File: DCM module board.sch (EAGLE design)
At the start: 2 parts

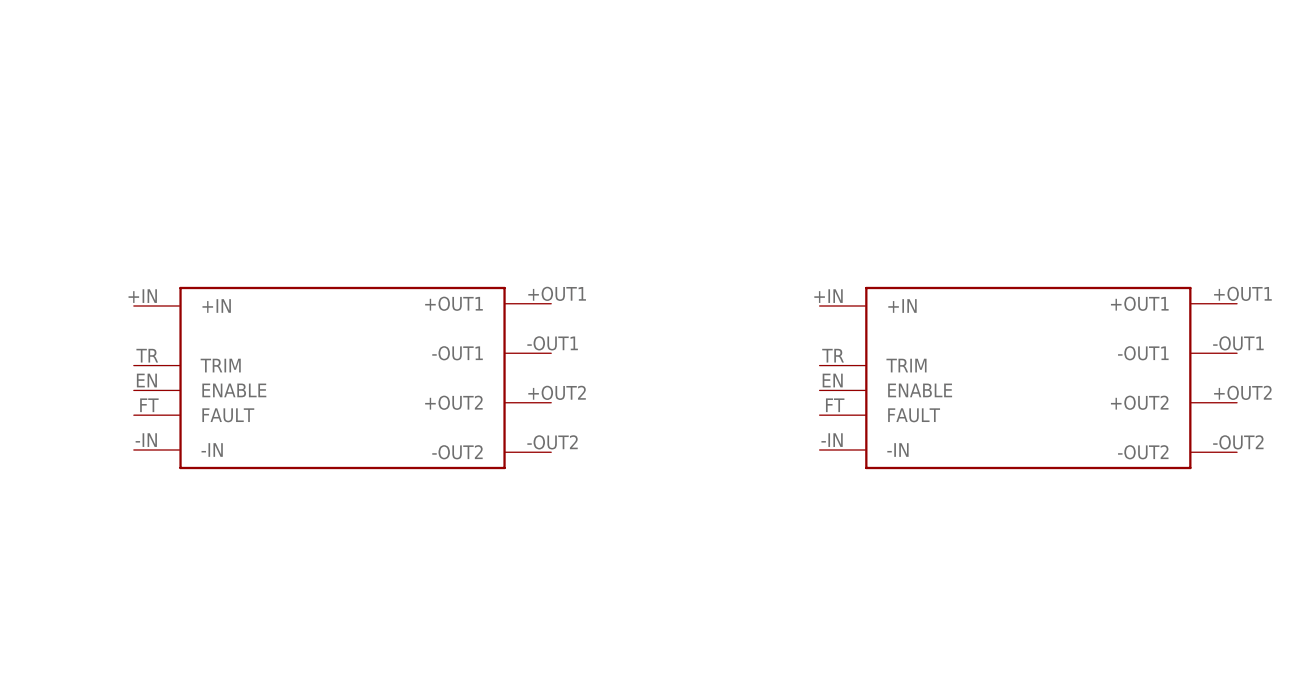
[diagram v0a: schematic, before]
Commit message: Add files via upload
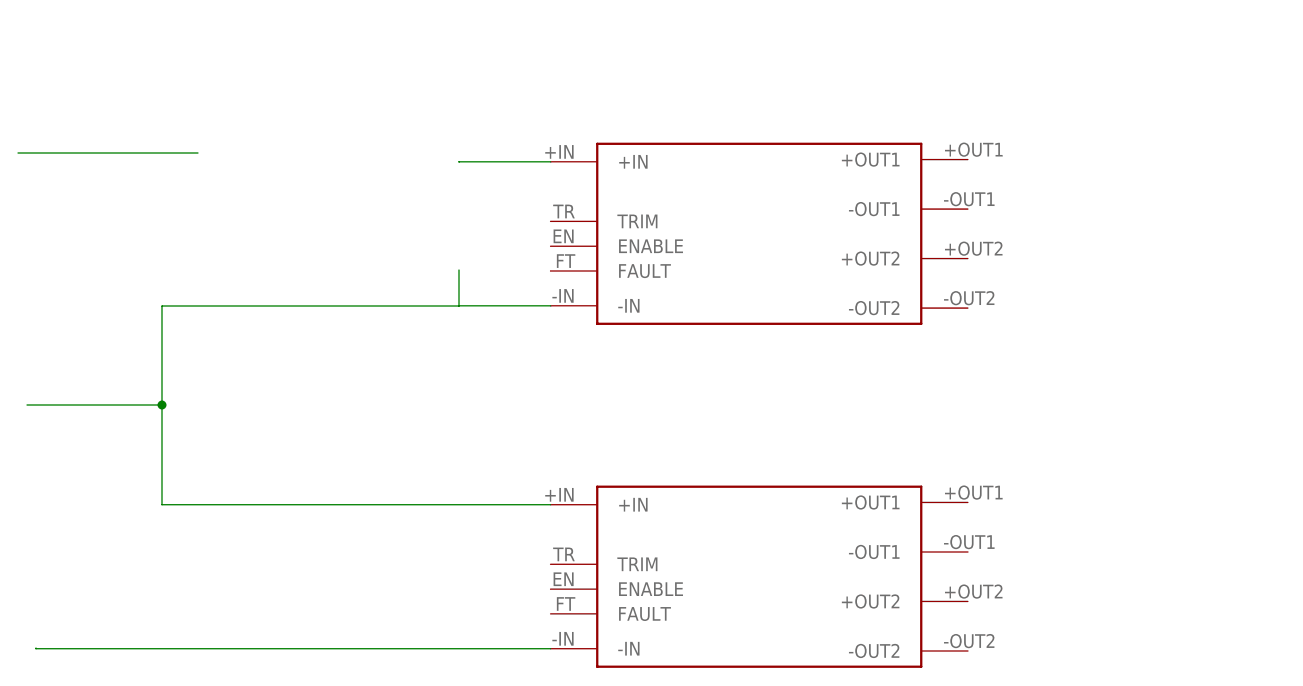
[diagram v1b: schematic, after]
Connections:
- new net N$1: U$1.+IN
- new net N$3: U$1.-IN
- new net N$4: U$2.+IN
- new net N$5: U$2.-IN
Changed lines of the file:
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@@
 <setting verticaltext="up"/>
 </settings>
-<grid distance="0.1" unitdist="inch" unit="inch" style="lines" multiple="1" display="no" altdistance="0.01" altunitdist="inch" altunit="inch"/>
+<grid distance="1" unitdist="mm" unit="mm" style="lines" multiple="1" display="yes" altdistance="0.01" altunitdist="inch" altunit="mm"/>
 <layers>
 <layer number="1" name="Top" color="4" fill="1" visible="no" active="no"/>
@@
 </plain>
 <instances>
-<instance part="U$1" gate="G$1" x="-27.94" y="0" smashed="yes"/>
-<instance part="U$2" gate="G$1" x="48.26" y="0" smashed="yes"/>
+<instance part="U$1" gate="G$1" x="18.36" y="16.02" smashed="yes"/>
+<instance part="U$2" gate="G$1" x="18.36" y="-22.08" smashed="yes"/>
 </instances>
 <busses>
 </busses>
 <nets>
+<net name="N$1" class="0">
+<segment>
+<pinref part="U$1" gate="G$1" pin="+IN"/>
+<wire x1="-4.83" y1="24.02" x2="-15" y2="24.02" width="0.1524" layer="91"/>
+<wire x1="-15" y1="24.02" x2="-15" y2="24" width="0.1524" layer="91"/>
+</segment>
+</net>
+<net name="N$2" class="0">
+<segment>
+<wire x1="-44" y1="25" x2="-64" y2="25" width="0.1524" layer="91"/>
+</segment>
+</net>
+<net name="N$3" class="0">
+<segment>
+<pinref part="U$1" gate="G$1" pin="-IN"/>
+<wire x1="-4.83" y1="8.02" x2="-15" y2="8.02" width="0.1524" layer="91"/>
+<wire x1="-15" y1="8.02" x2="-15" y2="12" width="0.1524" layer="91"/>
+</segment>
+</net>
+<net name="N$4" class="0">
+<segment>
+<wire x1="-15" y1="8" x2="-48" y2="8" width="0.1524" layer="91"/>
+<wire x1="-48" y1="8" x2="-48" y2="-3" width="0.1524" layer="91"/>
+<pinref part="U$2" gate="G$1" pin="+IN"/>
+<wire x1="-48" y1="-3" x2="-48" y2="-14.08" width="0.1524" layer="91"/>
+<wire x1="-48" y1="-14.08" x2="-4.83" y2="-14.08" width="0.1524" layer="91"/>
+<wire x1="-48" y1="-3" x2="-63" y2="-3" width="0.1524" layer="91"/>
+<junction x="-48" y="-3"/>
+</segment>
+</net>
+<net name="N$5" class="0">
+<segment>
+<pinref part="U$2" gate="G$1" pin="-IN"/>
+<wire x1="-4.83" y1="-30.08" x2="-62" y2="-30.08" width="0.1524" layer="91"/>
+<wire x1="-62" y1="-30.08" x2="-62" y2="-30" width="0.1524" layer="91"/>
+</segment>
+</net>
 </nets>
 </sheet>

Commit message: Add files via upload
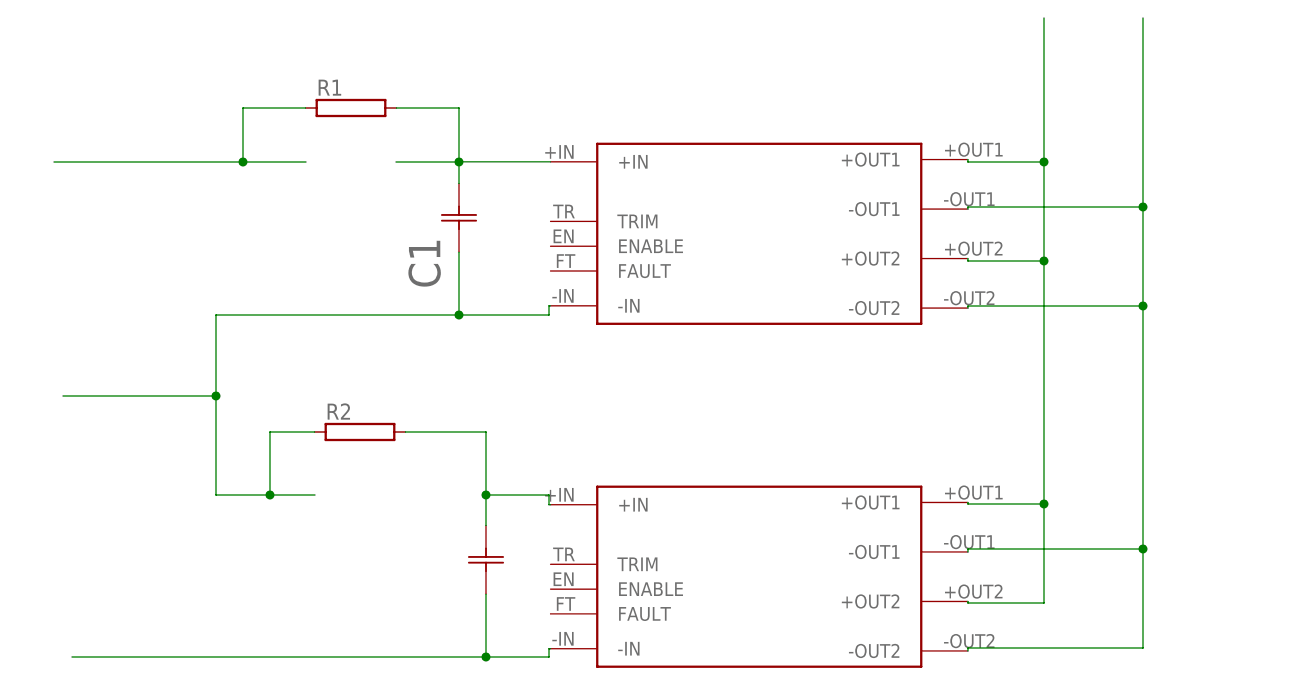
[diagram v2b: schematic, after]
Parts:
- added C1, C2: (no value), capacitor-emi:B58035U5305M062
- added R1, R2: (no value), resistor-power:RMG100-H
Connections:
- removed net N$4: U$2.+IN
- new net N$2: C2.2, R2.2, U$2.+IN
- new net N$6: U$1.-OUT1, U$1.-OUT2, U$2.-OUT1, U$2.-OUT2
- new net N$7: R1.1
- new net N$8: U$1.+OUT1, U$1.+OUT2, U$2.+OUT1, U$2.+OUT2
- net N$1: now also C1.2, R1.2
- net N$3: now also C2.1, U$2.-IN; no longer U$1.-IN
- net N$5: now also C1.1, R2.1, U$1.-IN; no longer U$2.-IN
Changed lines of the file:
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@@
 <setting verticaltext="up"/>
 </settings>
-<grid distance="1" unitdist="mm" unit="mm" style="lines" multiple="1" display="yes" altdistance="0.01" altunitdist="inch" altunit="mm"/>
+<grid distance="1" unitdist="mm" unit="mm" style="lines" multiple="1" display="yes" altdistance="0.1" altunitdist="mm" altunit="mm"/>
 <layers>
 <layer number="1" name="Top" color="4" fill="1" visible="no" active="no"/>
@@
 <part name="U$1" library="dc-dc-converter" library_urn="urn:adsk.eagle:library:24542449" deviceset="DCM4623TD2N13C8T00" device="" package3d_urn="urn:adsk.eagle:package:24542464/2"/>
 <part name="U$2" library="dc-dc-converter" library_urn="urn:adsk.eagle:library:24542449" deviceset="DCM4623TD2N13C8T00" device="" package3d_urn="urn:adsk.eagle:package:24542464/2"/>
+<part name="R1" library="resistor-power" library_urn="urn:adsk.eagle:library:344" deviceset="RMG100" device="-H" package3d_urn="urn:adsk.eagle:package:25183/1"/>
+<part name="R2" library="resistor-power" library_urn="urn:adsk.eagle:library:344" deviceset="RMG100" device="-H" package3d_urn="urn:adsk.eagle:package:25183/1"/>
+<part name="C1" library="capacitor-emi" library_urn="urn:adsk.eagle:library:24583833" deviceset="B58035U5305M062" device="" package3d_urn="urn:adsk.eagle:package:24583837/1"/>
+<part name="C2" library="capacitor-emi" library_urn="urn:adsk.eagle:library:24583833" deviceset="B58035U5305M062" device="" package3d_urn="urn:adsk.eagle:package:24583837/1"/>
 </parts>
 <sheets>
@@
 <instance part="U$1" gate="G$1" x="18.36" y="16.02" smashed="yes"/>
 <instance part="U$2" gate="G$1" x="18.36" y="-22.08" smashed="yes"/>
+<instance part="R1" gate="G$1" x="-27" y="30" smashed="yes">
+<attribute name="NAME" x="-30.81" y="31.3716" size="1.778" layer="95"/>
+<attribute name="VALUE" x="-30.81" y="27.079" size="1.778" layer="96"/>
+</instance>
+<instance part="R2" gate="G$1" x="-26" y="-6" smashed="yes">
+<attribute name="NAME" x="-29.81" y="-4.6284" size="1.778" layer="95"/>
+<attribute name="VALUE" x="-29.81" y="-8.921" size="1.778" layer="96"/>
+</instance>
+<instance part="C1" gate="A" x="-15" y="14" smashed="yes" rot="R90">
+<attribute name="VALUE" x="-9.4628" y="8.8438" size="3.4798" layer="96" ratio="10" rot="SR90"/>
+<attribute name="NAME" x="-17.0828" y="9.9106" size="3.4798" layer="95" ratio="10" rot="SR90"/>
+</instance>
+<instance part="C2" gate="A" x="-12" y="-24" smashed="yes" rot="R90">
+<attribute name="VALUE" x="-6.4628" y="-29.1562" size="3.4798" layer="96" ratio="10" rot="SR90"/>
+</instance>
 </instances>
 <busses>
@@
 <pinref part="U$1" gate="G$1" pin="+IN"/>
 <wire x1="-4.83" y1="24.02" x2="-15" y2="24.02" width="0.1524" layer="91"/>
+<wire x1="-15" y1="24.02" x2="-15" y2="30" width="0.1524" layer="91"/>
+<pinref part="R1" gate="G$1" pin="2"/>
+<wire x1="-15" y1="30" x2="-21.92" y2="30" width="0.1524" layer="91"/>
+<pinref part="C1" gate="A" pin="2"/>
 <wire x1="-15" y1="24.02" x2="-15" y2="24" width="0.1524" layer="91"/>
+<wire x1="-15" y1="24" x2="-15" y2="21.62" width="0.1524" layer="91"/>
+<wire x1="-15" y1="24" x2="-22" y2="24" width="0.1524" layer="91"/>
+<junction x="-15" y="24"/>
+</segment>
+</net>
+<net name="N$8" class="0">
+<segment>
+<pinref part="U$2" gate="G$1" pin="+OUT2"/>
+<wire x1="50" y1="24" x2="50" y2="13" width="0.1524" layer="91"/>
+<wire x1="50" y1="13" x2="50" y2="-14" width="0.1524" layer="91"/>
+<wire x1="50" y1="-14" x2="50" y2="-25" width="0.1524" layer="91"/>
+<wire x1="50" y1="-25" x2="41.55" y2="-25" width="0.1524" layer="91"/>
+<wire x1="41.55" y1="-25" x2="41.55" y2="-24.83" width="0.1524" layer="91"/>
+<pinref part="U$2" gate="G$1" pin="+OUT1"/>
+<wire x1="41.55" y1="-13.83" x2="41.55" y2="-14" width="0.1524" layer="91"/>
+<wire x1="41.55" y1="-14" x2="50" y2="-14" width="0.1524" layer="91"/>
+<junction x="50" y="-14"/>
+<pinref part="U$1" gate="G$1" pin="+OUT2"/>
+<wire x1="41.55" y1="13.27" x2="41.55" y2="13" width="0.1524" layer="91"/>
+<wire x1="41.55" y1="13" x2="50" y2="13" width="0.1524" layer="91"/>
+<junction x="50" y="13"/>
+<pinref part="U$1" gate="G$1" pin="+OUT1"/>
+<wire x1="41.55" y1="24.27" x2="41.55" y2="24" width="0.1524" layer="91"/>
+<wire x1="41.55" y1="24" x2="50" y2="24" width="0.1524" layer="91"/>
+<junction x="50" y="24"/>
+<wire x1="50" y1="24" x2="50" y2="40" width="0.1524" layer="91"/>
+</segment>
+</net>
+<net name="N$6" class="0">
+<segment>
+<wire x1="61" y1="-30" x2="61" y2="-19" width="0.1524" layer="91"/>
+<pinref part="U$2" gate="G$1" pin="-OUT2"/>
+<wire x1="61" y1="-19" x2="61" y2="8" width="0.1524" layer="91"/>
+<wire x1="61" y1="8" x2="61" y2="19" width="0.1524" layer="91"/>
+<wire x1="61" y1="19" x2="61" y2="40" width="0.1524" layer="91"/>
+<wire x1="41.55" y1="-30.33" x2="41.55" y2="-30" width="0.1524" layer="91"/>
+<wire x1="41.55" y1="-30" x2="61" y2="-30" width="0.1524" layer="91"/>
+<pinref part="U$2" gate="G$1" pin="-OUT1"/>
+<wire x1="41.55" y1="-19.33" x2="41.55" y2="-19" width="0.1524" layer="91"/>
+<wire x1="41.55" y1="-19" x2="61" y2="-19" width="0.1524" layer="91"/>
+<junction x="61" y="-19"/>
+<pinref part="U$1" gate="G$1" pin="-OUT2"/>
+<wire x1="41.55" y1="7.77" x2="41.55" y2="8" width="0.1524" layer="91"/>
+<wire x1="41.55" y1="8" x2="61" y2="8" width="0.1524" layer="91"/>
+<junction x="61" y="8"/>
+<pinref part="U$1" gate="G$1" pin="-OUT1"/>
+<wire x1="41.55" y1="18.77" x2="41.55" y2="19" width="0.1524" layer="91"/>
+<wire x1="41.55" y1="19" x2="61" y2="19" width="0.1524" layer="91"/>
+<junction x="61" y="19"/>
 </segment>
 </net>
 <net name="N$2" class="0">
 <segment>
-<wire x1="-44" y1="25" x2="-64" y2="25" width="0.1524" layer="91"/>
+<pinref part="U$2" gate="G$1" pin="+IN"/>
+<wire x1="-4.83" y1="-14.08" x2="-5" y2="-14.08" width="0.1524" layer="91"/>
+<wire x1="-5" y1="-14.08" x2="-5" y2="-13" width="0.1524" layer="91"/>
+<wire x1="-5" y1="-13" x2="-12" y2="-13" width="0.1524" layer="91"/>
+<pinref part="C2" gate="A" pin="2"/>
+<wire x1="-12" y1="-13" x2="-12" y2="-16.38" width="0.1524" layer="91"/>
+<junction x="-12" y="-13"/>
+<pinref part="R2" gate="G$1" pin="2"/>
+<wire x1="-12" y1="-13" x2="-12" y2="-6" width="0.1524" layer="91"/>
+<wire x1="-12" y1="-6" x2="-20.92" y2="-6" width="0.1524" layer="91"/>
+</segment>
+</net>
+<net name="N$5" class="0">
+<segment>
+<pinref part="U$1" gate="G$1" pin="-IN"/>
+<wire x1="-4.83" y1="8.02" x2="-5" y2="8.02" width="0.1524" layer="91"/>
+<wire x1="-5" y1="8.02" x2="-5" y2="7" width="0.1524" layer="91"/>
+<wire x1="-5" y1="7" x2="-15" y2="7" width="0.1524" layer="91"/>
+<pinref part="C1" gate="A" pin="1"/>
+<wire x1="-15" y1="7" x2="-15" y2="14" width="0.1524" layer="91"/>
+<wire x1="-15" y1="7" x2="-42" y2="7" width="0.1524" layer="91"/>
+<junction x="-15" y="7"/>
+<wire x1="-42" y1="7" x2="-42" y2="-2" width="0.1524" layer="91"/>
+<wire x1="-42" y1="-2" x2="-42" y2="-13" width="0.1524" layer="91"/>
+<wire x1="-36" y1="-13" x2="-31" y2="-13" width="0.1524" layer="91"/>
+<wire x1="-36" y1="-6" x2="-36" y2="-13" width="0.1524" layer="91"/>
+<pinref part="R2" gate="G$1" pin="1"/>
+<wire x1="-31.08" y1="-6" x2="-36" y2="-6" width="0.1524" layer="91"/>
+<wire x1="-42" y1="-13" x2="-36" y2="-13" width="0.1524" layer="91"/>
+<junction x="-36" y="-13"/>
+<wire x1="-42" y1="-2" x2="-59" y2="-2" width="0.1524" layer="91"/>
+<junction x="-42" y="-2"/>
+</segment>
+</net>
+<net name="N$7" class="0">
+<segment>
+<pinref part="R1" gate="G$1" pin="1"/>
+<wire x1="-32.08" y1="30" x2="-39" y2="30" width="0.1524" layer="91"/>
+<wire x1="-39" y1="30" x2="-39" y2="24" width="0.1524" layer="91"/>
+<wire x1="-32" y1="24" x2="-39" y2="24" width="0.1524" layer="91"/>
+<wire x1="-39" y1="24" x2="-60" y2="24" width="0.1524" layer="91"/>
+<junction x="-39" y="24"/>
 </segment>
 </net>
 <net name="N$3" class="0">
 <segment>
-<pinref part="U$1" gate="G$1" pin="-IN"/>
-<wire x1="-4.83" y1="8.02" x2="-15" y2="8.02" width="0.1524" layer="91"/>
-<wire x1="-15" y1="8.02" x2="-15" y2="12" width="0.1524" layer="91"/>
-</segment>
-</net>
-<net name="N$4" class="0">
-<segment>
-<wire x1="-15" y1="8" x2="-48" y2="8" width="0.1524" layer="91"/>
-<wire x1="-48" y1="8" x2="-48" y2="-3" width="0.1524" layer="91"/>
-<pinref part="U$2" gate="G$1" pin="+IN"/>
-<wire x1="-48" y1="-3" x2="-48" y2="-14.08" width="0.1524" layer="91"/>
-<wire x1="-48" y1="-14.08" x2="-4.83" y2="-14.08" width="0.1524" layer="91"/>
-<wire x1="-48" y1="-3" x2="-63" y2="-3" width="0.1524" layer="91"/>
-<junction x="-48" y="-3"/>
-</segment>
-</net>
-<net name="N$5" class="0">
-<segment>
 <pinref part="U$2" gate="G$1" pin="-IN"/>
-<wire x1="-4.83" y1="-30.08" x2="-62" y2="-30.08" width="0.1524" layer="91"/>
-<wire x1="-62" y1="-30.08" x2="-62" y2="-30" width="0.1524" layer="91"/>
-</segment>
-</net>
+<wire x1="-4.83" y1="-30.08" x2="-5" y2="-30.08" width="0.1524" layer="91"/>
+<wire x1="-5" y1="-30.08" x2="-5" y2="-31" width="0.1524" layer="91"/>
+<wire x1="-5" y1="-31" x2="-12" y2="-31" width="0.1524" layer="91"/>
+<pinref part="C2" gate="A" pin="1"/>
+<wire x1="-12" y1="-31" x2="-12" y2="-24" width="0.1524" layer="91"/>
+<junction x="-12" y="-31"/>
+<wire x1="-12" y1="-31" x2="-58" y2="-31" width="0.1524" layer="91"/>
+</segment>
+</net>
